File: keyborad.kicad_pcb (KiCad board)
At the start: 2 copper layers, 27 parts, among them P1 1pin, P10 1pin, P11 1pin, P12 1pin, P13 1pin, P2 1pin, P3 1pin, P4 1pin, P5 1pin, P6 1pin, P7 1pin, P8 1pin, P9 1pin, SW1 SW_DIP_x01, SW2 SW_DIP_x01, SW3 SW_DIP_x01, SW4 SW_DIP_x01, SW5 SW_DIP_x01, SW6 SW_DIP_x01

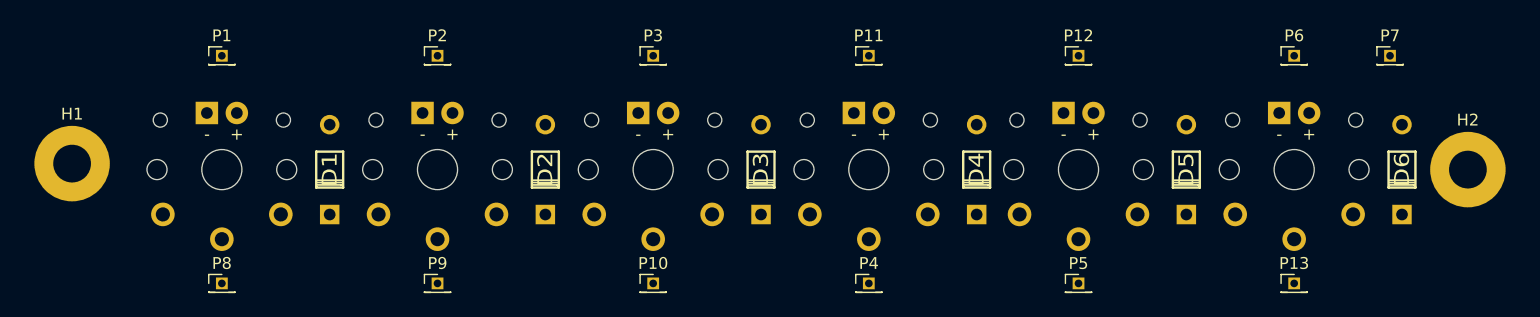
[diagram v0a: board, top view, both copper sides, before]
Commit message: とりあえず形にした
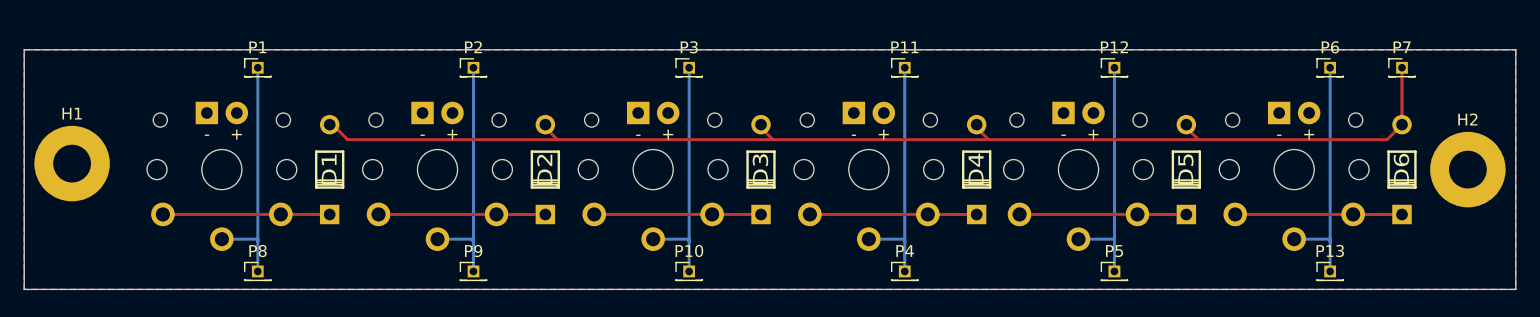
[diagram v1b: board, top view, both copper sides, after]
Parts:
- moved P1 3.21 mm to (125.0, 65.0)
- moved P11 3.21 mm to (179.8, 65.0)
- moved P12 3.21 mm to (197.6, 65.0)
- moved P2 3.21 mm to (143.3, 65.0)
- moved P3 3.21 mm to (161.5, 65.0)
- moved P6 3.21 mm to (215.9, 65.0)
- moved P10 3.21 mm to (161.5, 82.3)
- moved P13 3.21 mm to (215.9, 82.3)
- moved P4 3.21 mm to (179.8, 82.3)
- moved P5 3.21 mm to (197.6, 82.3)
- moved P8 3.21 mm to (125.0, 82.3)
- moved P9 3.21 mm to (143.3, 82.3)
- moved P7 1.44 mm to (222.0, 65.0)
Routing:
- net row0: track 0.00 -> 103.6 mm
- net col5: track 0.00 -> 20.5 mm
- net col4: track 0.00 -> 20.5 mm
- net col3: track 0.00 -> 20.5 mm
- net col2: track 0.00 -> 20.5 mm
- net col0: track 0.00 -> 20.5 mm
- net col1: track 0.00 -> 20.4 mm
- net Net-(D6-Pad2): track 0.00 -> 14.1 mm
- net Net-(D2-Pad2): track 0.00 -> 14.1 mm
- net Net-(D5-Pad2): track 0.00 -> 14.1 mm
- net Net-(D4-Pad2): track 0.00 -> 14.1 mm
- net Net-(D1-Pad2): track 0.00 -> 14.1 mm
- net Net-(D3-Pad2): track 0.00 -> 14.1 mm
- added copper zone on B.Cu, net (none)
- added copper zone on F.Cu, net (none)
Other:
- board outline added: 126.5 x 20.3 mm
